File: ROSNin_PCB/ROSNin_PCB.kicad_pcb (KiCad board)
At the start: 2 copper layers, 1 part, among them U1 Tang_Nano_20K

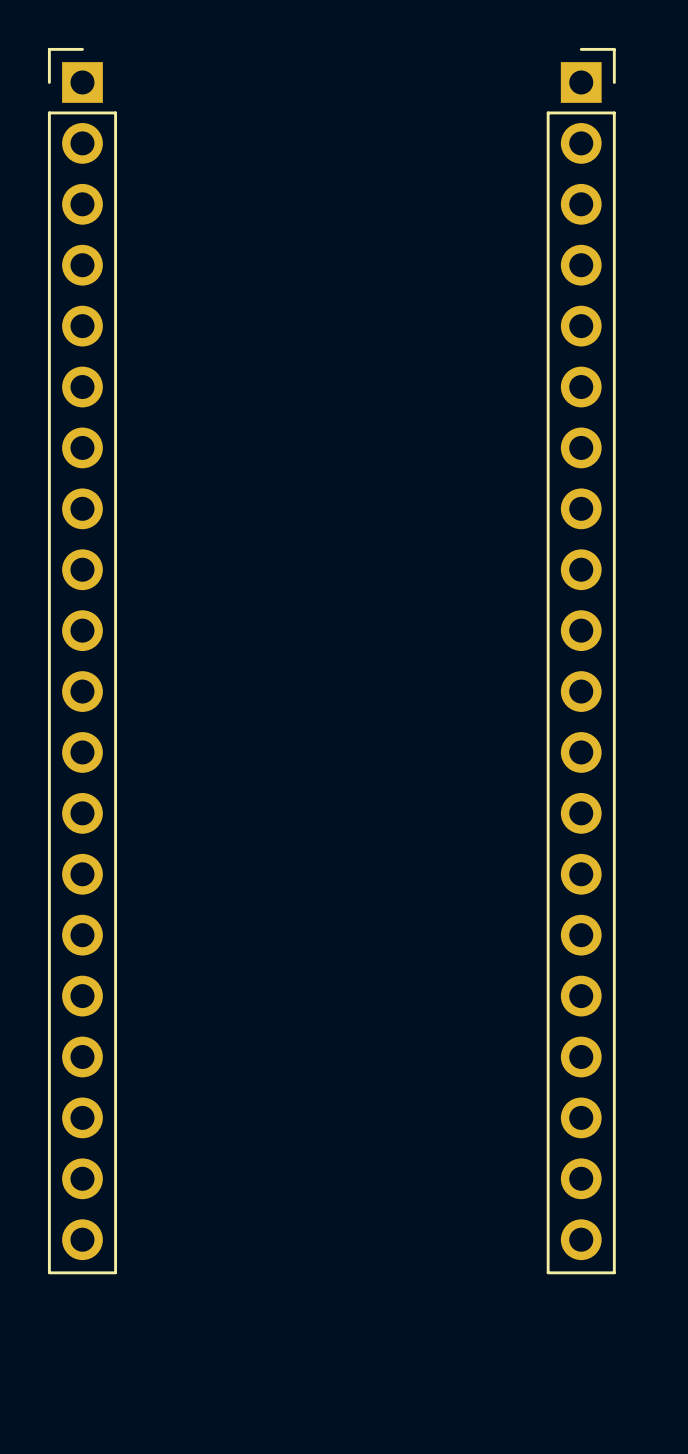
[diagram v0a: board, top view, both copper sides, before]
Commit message: feat: add Tang Nano 20K library for the project
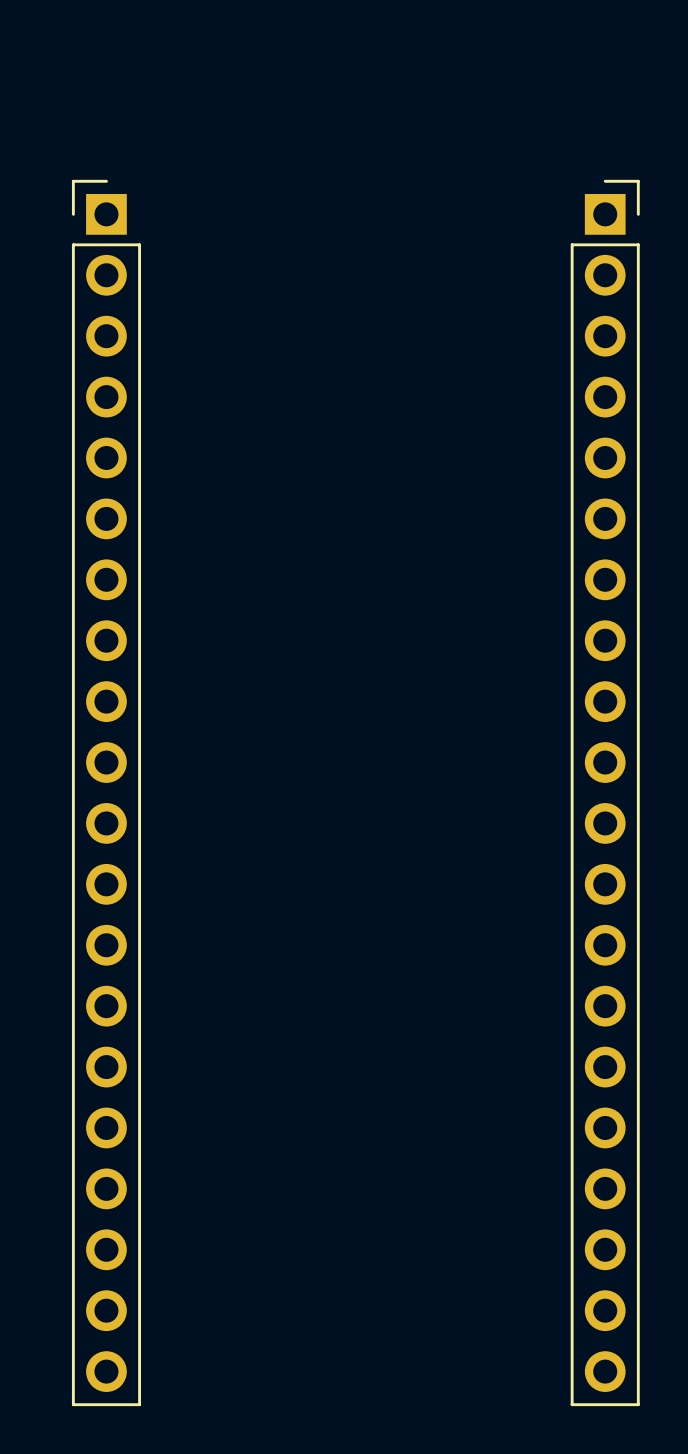
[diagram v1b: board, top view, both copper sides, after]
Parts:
- moved U1 5.59 mm to (135.2, 74.2)
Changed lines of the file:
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@@
 	(footprint "Custom:TangNano_20K"
 		(layer "F.Cu")
-		(at 134.2 68.74)
+		(at 135.2 74.24)
 		(property "Reference" "U1"
 			(at 0 -2.38 0)
